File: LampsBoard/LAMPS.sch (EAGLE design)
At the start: 41 parts, among them IC1 LM358N, IC2 LM358N, IC3 5V, Q1 TIP120

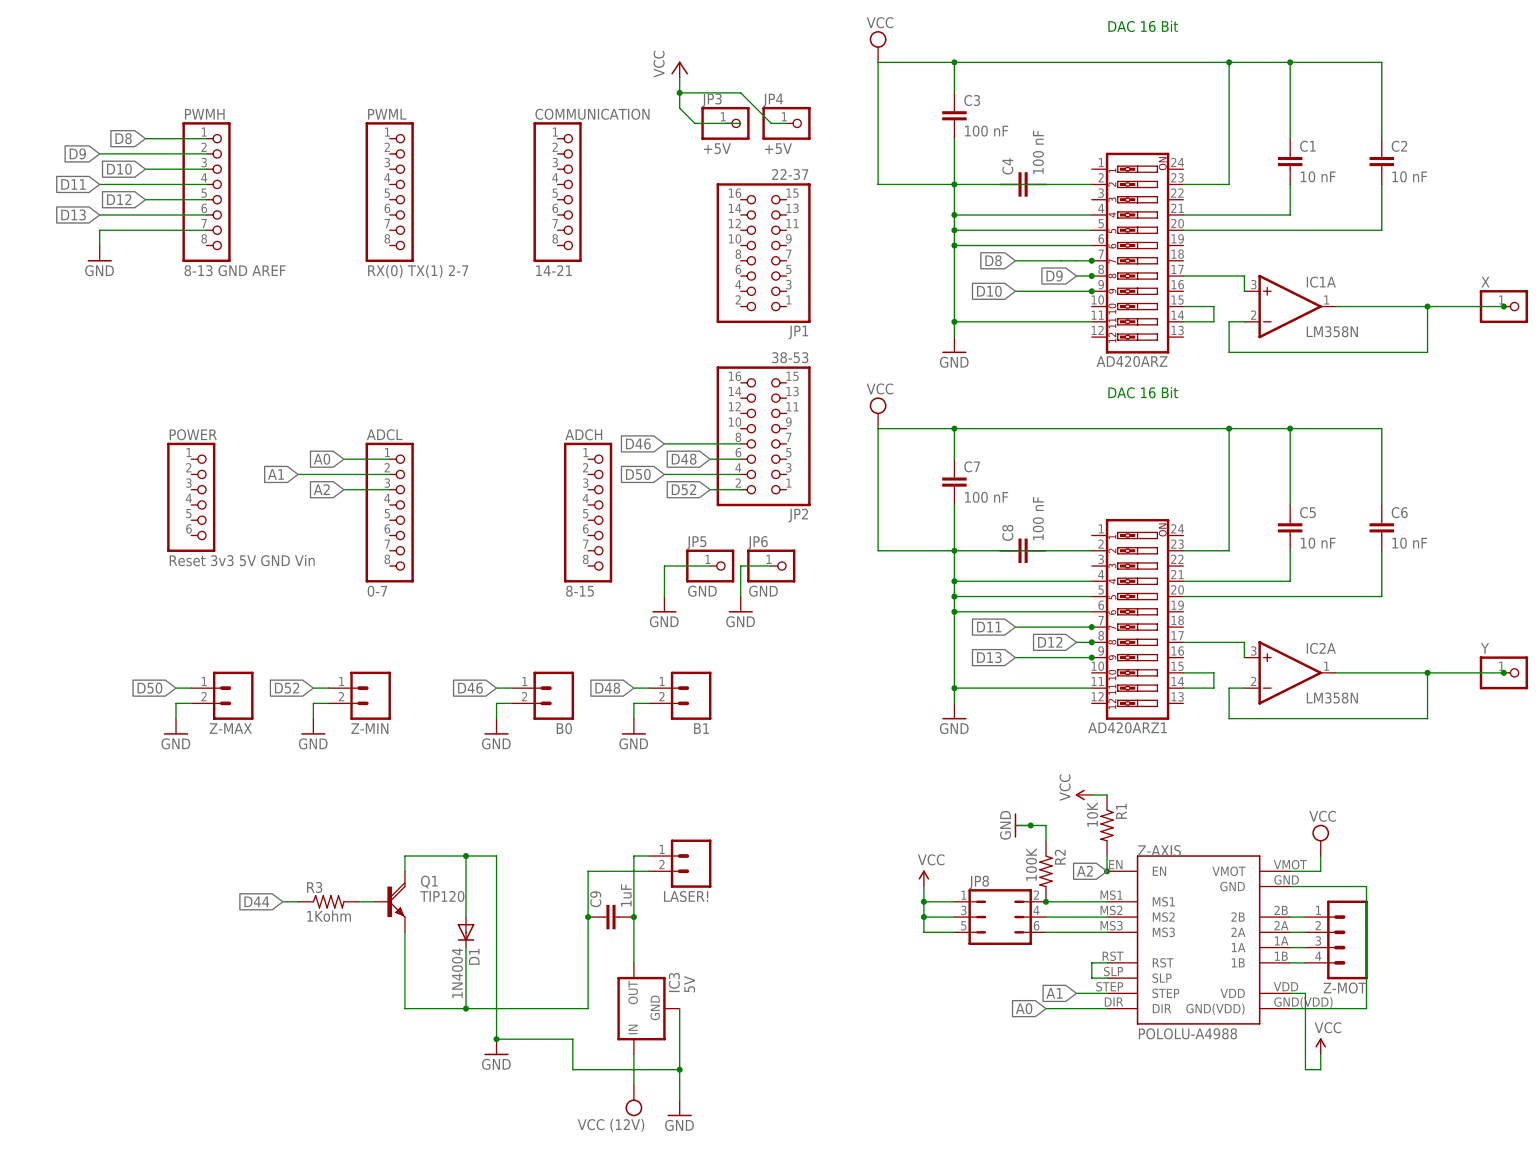
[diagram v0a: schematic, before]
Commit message: Clean up
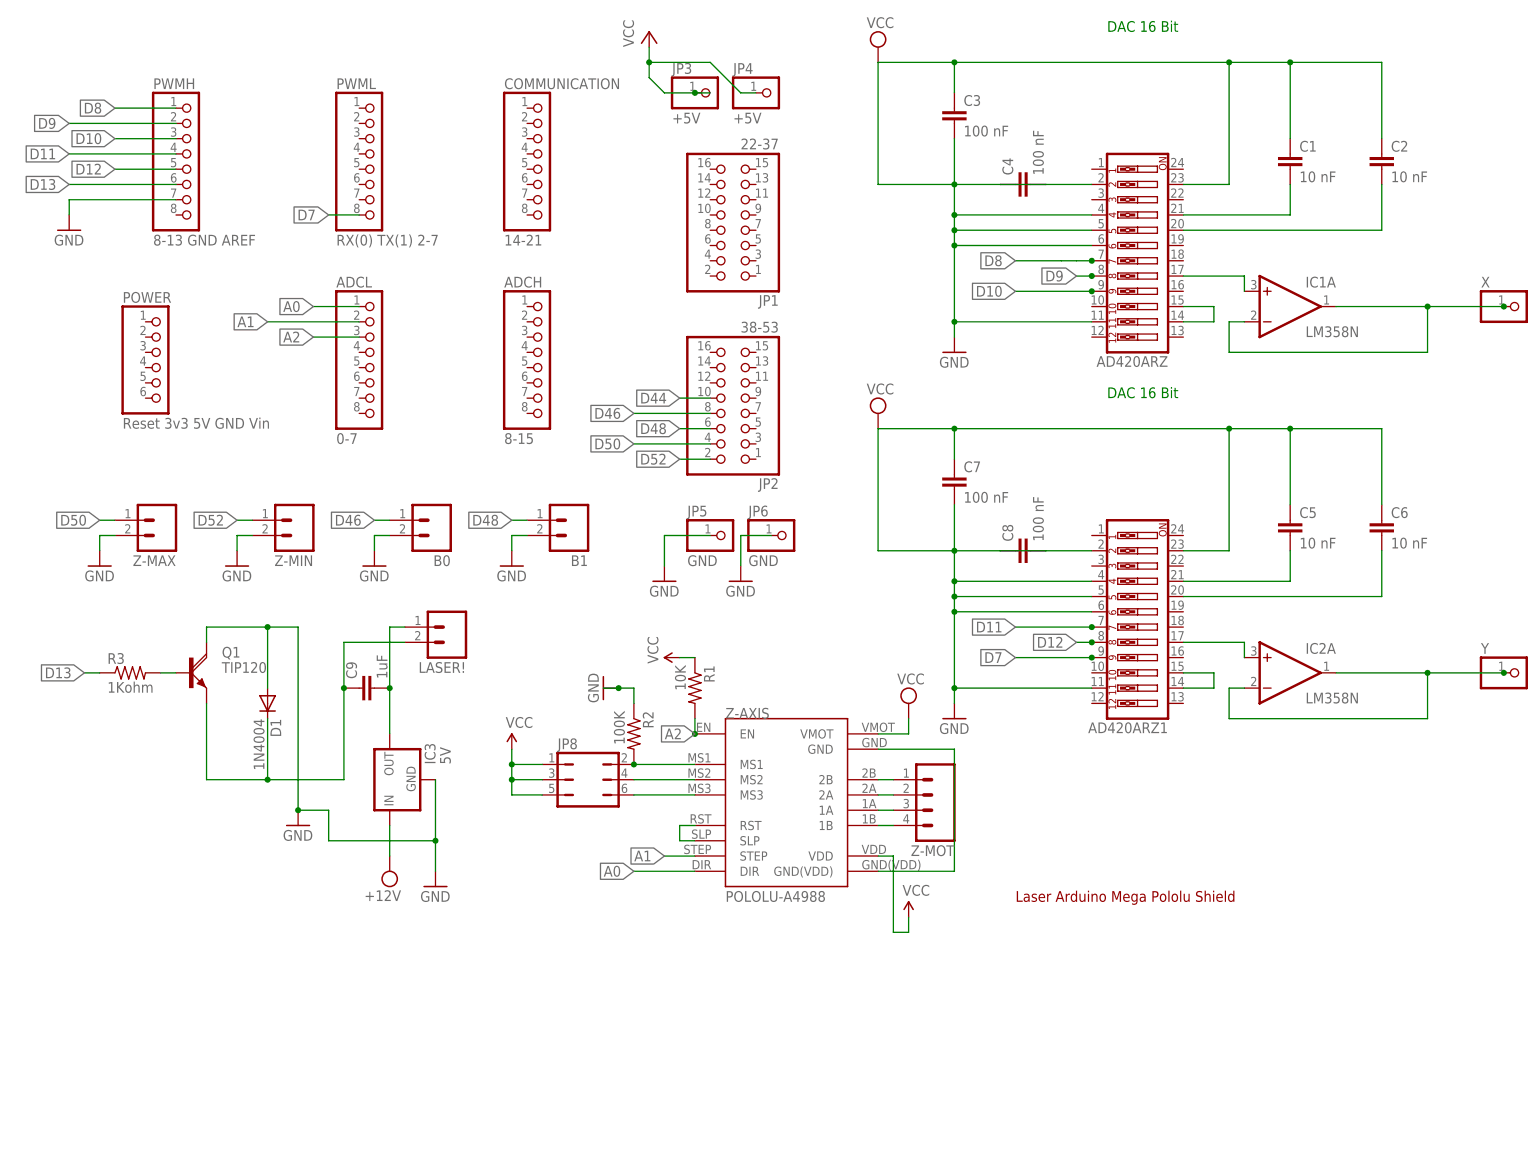
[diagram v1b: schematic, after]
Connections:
- new net D7: AD420ARZ1.9, PWML.8
- net D13: now also R3.1; no longer AD420ARZ1.9
- net D44: now also JP2.10; no longer R3.1
- net VCC: now also JP3.1
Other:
- note added: "Laser Arduino Mega Pololu Shield"
- moved on the sheet: ADCH, ADCL, B0, B1, C9, COMMUNICATION, D1, IC3, JP1, JP2, JP3, JP4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
